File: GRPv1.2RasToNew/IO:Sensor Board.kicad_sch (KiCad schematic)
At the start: 20 parts, among them J1 B3B-XH-A, J3 B6B-XH-A, J4 B2B-XH-A, U1 BMP581, U2 ESP32-S3-DEVKITC-1-N8R2, U3 TPS79333-EP, U4 ICM-20948, U5 TPS79318-EP

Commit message: teensy modification
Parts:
- removed Module1: ComputeModule4-CM4, CM4IO:Raspberry-Pi-4-Compute-Module, symbol CM4IO:ComputeModule4-CM4
- removed U2: ESP32-S3-DEVKITC-1-N8R2, ESP32-S3-DEVKITC-1-N8R2:XCVR_ESP32-S3-DEVKITC-1-N8R2, symbol ESP32-S3-DEVKITC-1-N8R2:ESP32-S3-DEVKITC-1-N8R2
- added U6: Teensy4.1, modFiles:Teensy41, symbol teensy:Teensy4.1
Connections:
- net +5V: now also U6.48 (VIN)
- net BMP_CLK: now also U6.19 (27_A13_SCK1)
- net BMP_CS: now also U6.2 (0_RX1_CRX2_CS1)
- net BMP_MISO: now also U6.3 (1_TX1_CTX2_MISO1)
- net BMP_MOSI: now also U6.18 (26_A12_MOSI1)
- net GND: now also U6.1 (GND), U6.34 (GND), U6.47 (GND), U6.52 (GND), U6.58 (GND), U6.59 (GND), U6.64 (GND)
- net ICM_CLK: now also U6.35 (13_SCK_LED)
- net ICM_CS: now also U6.29 (37_CS)
- net ICM_MISO: now also U6.14 (12_MISO_MQSL)
- net ICM_MOSI: now also U6.13 (11_MOSI_CTX1)
- net PYRO_1: now also U6.27 (35_TX8)
- net PYRO_2: now also U6.26 (34_RX8)
- net PYRO_3: now also U6.25 (33_MCLK2)
- net PYRO_4: now also U6.39 (17_A3_TX4_SDA1)
- net PYRO_5: now also U6.38 (16_A2_RX4_SCL1)
- net SERVO_1: now also U6.45 (23_A9_CRX1_MCLK1)
- net SERVO_2: now also U6.44 (22_A8_CTX1)
- net SERVO_3: now also U6.41 (19_A5_SCL)
- net SERVO_4: now also U6.40 (18_A4_SDA)

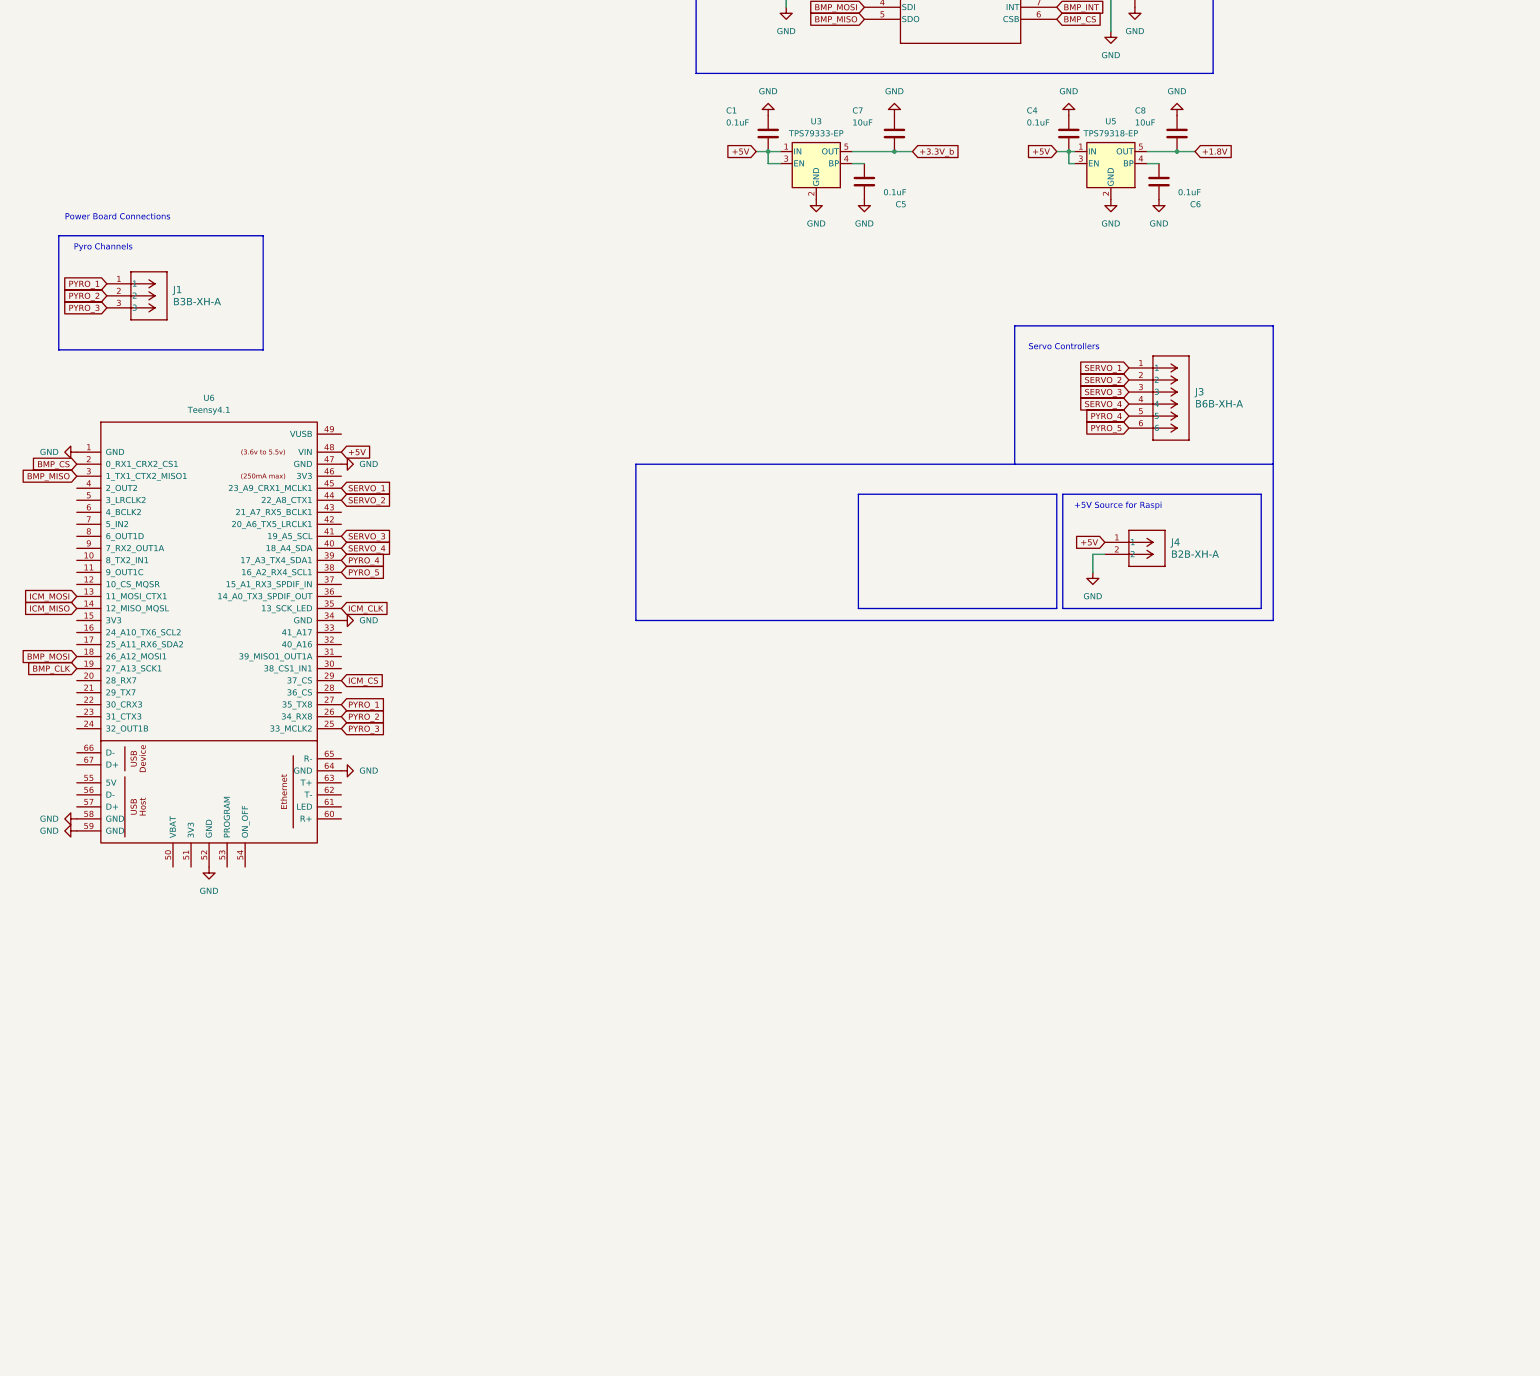
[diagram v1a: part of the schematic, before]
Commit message: esp switch 1
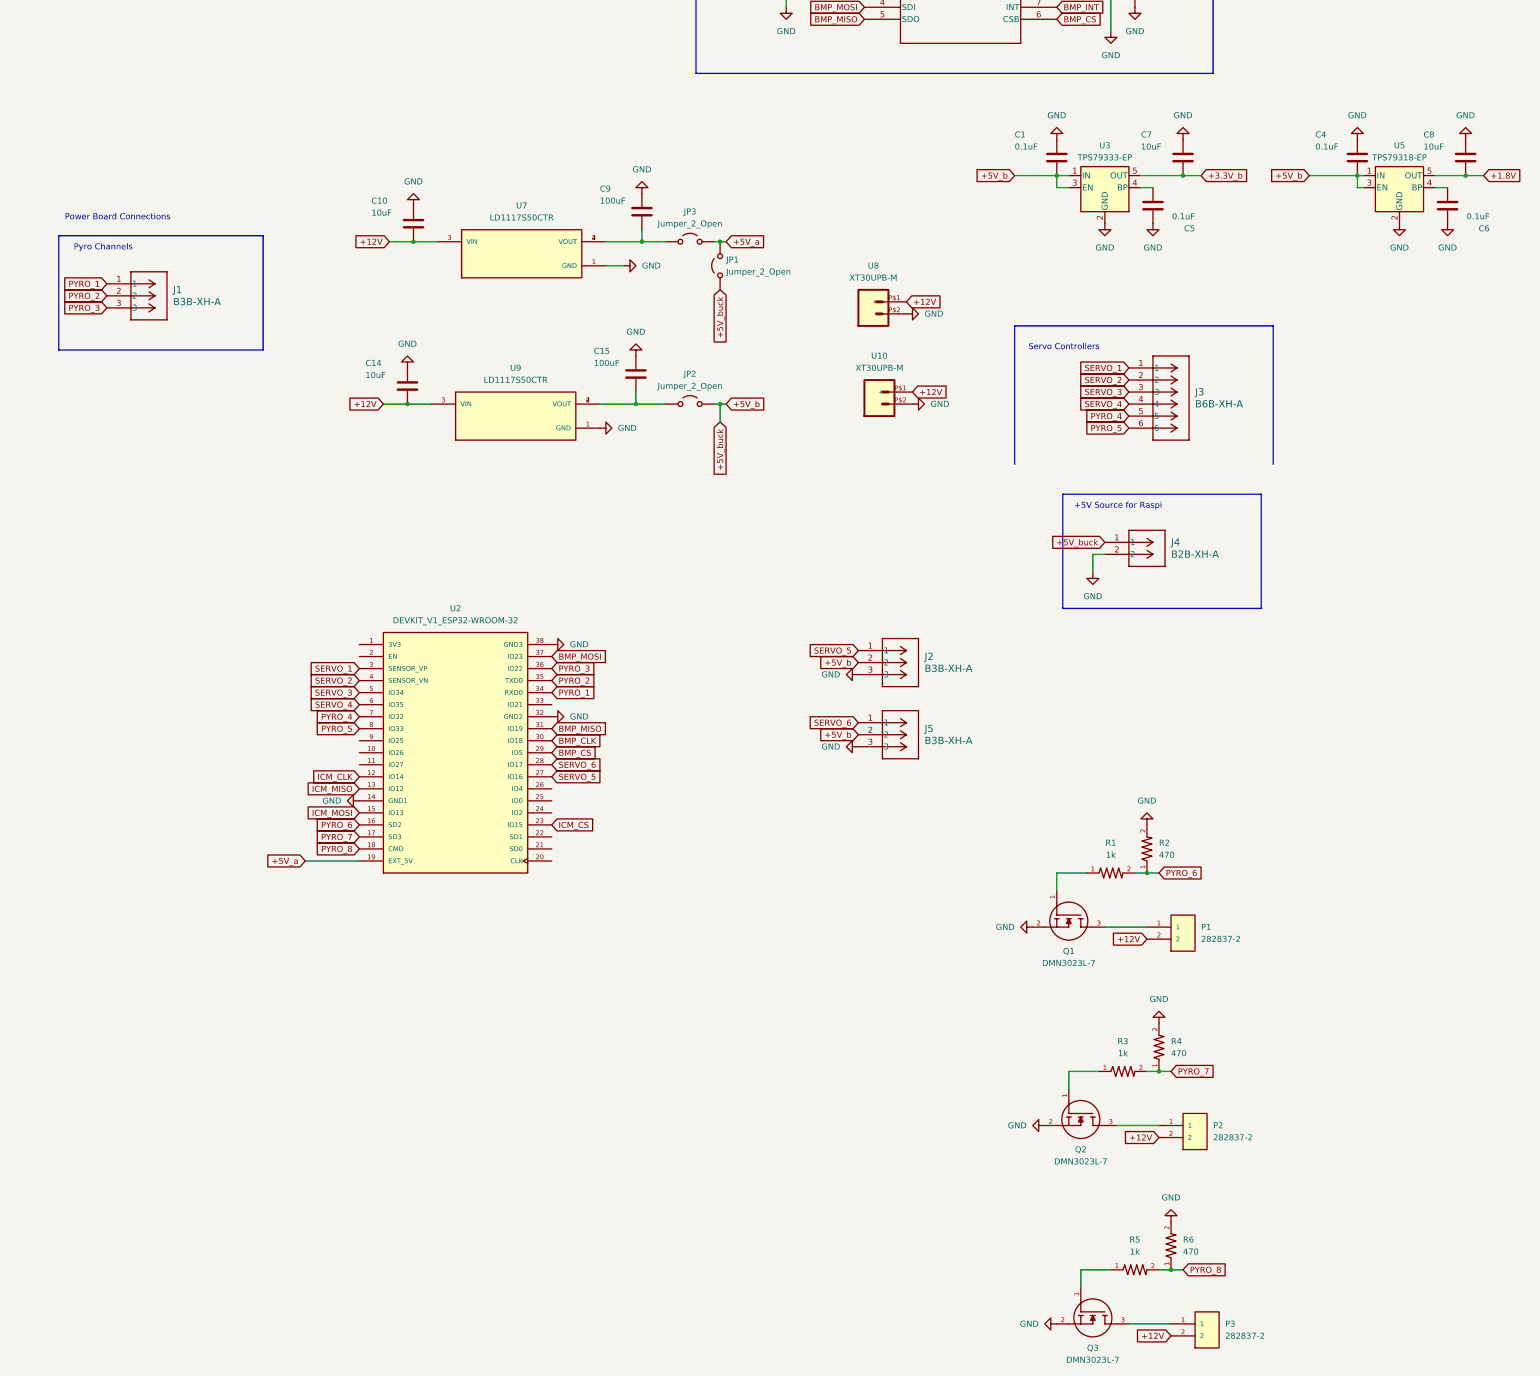
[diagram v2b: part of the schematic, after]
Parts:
- removed U6: Teensy4.1, modFiles:Teensy41, symbol teensy:Teensy4.1
- added C10, C14: 10uF, Capacitors:C_0805_2012Metric_Pad1.18x1.45mm_HandSolder, symbol Device:C
- added C15, C9: 100uF, Capacitors:C_0805_2012Metric_Pad1.18x1.45mm_HandSolder, symbol Device:C
- added J2, J5: B3B-XH-A, B3B:CONN_B3B-XH-A_JST, symbol 2025-01-01_02-21-05:B3B-XH-A
- added JP1, JP2, JP3: Jumper_2_Open, Jumper:SolderJumper-2_P1.3mm_Open_RoundedPad1.0x1.5mm, symbol Jumper:Jumper_2_Open
- added P1, P2, P3: 282837-2, ScrewTerminal:CUI_TB002-500-02BE, symbol 282837-2:282837-2
- added Q1, Q2, Q3: DMN3023L-7, FETS:SOT96P240X100-3N, symbol DMN3023L-7:DMN3023L-7
- added R1, R3, R5: 1k, Resistor:R_0805_2012Metric_Pad1.20x1.40mm_HandSolder, symbol 8-2176243-2:8-2176243-2
- added R2, R4, R6: 470, Resistor:R_0805_2012Metric_Pad1.20x1.40mm_HandSolder, symbol 8-2176243-2:8-2176243-2
- added U10, U8: XT30UPB-M, XTConnectors:XT30UPB-M, symbol XT30UPB-M:XT30UPB-M
- added U2: DEVKIT_V1_ESP32-WROOM-32, esp32wroom:MODULE_DEVKIT_V1_ESP32-WROOM-32, symbol DEVKIT_V1_ESP32-WROOM-32:DEVKIT_V1_ESP32-WROOM-32
- added U7, U9: LD1117S50CTR, LD1117S50CTRlib:LD1117S50CTR, symbol LD1117S50CTR:LD1117S50CTR
- C1, C11, C12, C13, C2, C3, C4, C5, C6, C7, C8: footprint Capacitor_SMD:C_0805_2012Metric_Pad1.18x1.45mm_HandSolder -> Capacitors:C_0805_2012Metric_Pad1.18x1.45mm_HandSolder
- J1: footprint Connector_JST:JST_XH_B3B-XH-A_1x03_P2.50mm_Vertical -> B3B:CONN_B3B-XH-A_JST
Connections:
- net BMP_CLK: now also U2.30 (IO18)
- net BMP_CS: now also U2.29 (IO5)
- net BMP_MISO: now also U2.31 (IO19)
- net BMP_MOSI: now also U2.37 (IO23)
- net GND: now also C10.1, C14.1, C15.1, C9.1, J2.3, J5.3, Q1.2, Q2.2, Q3.2, R2.2, R4.2, R6.2, U10.P$2 (-), U2.14 (GND1), U2.32 (GND2), U2.38 (GND3), U7.1 (GND), U8.P$2 (-), U9.1 (GND)
- net ICM_CLK: now also U2.12 (IO14)
- net ICM_CS: now also U2.23 (IO15)
- net ICM_MISO: now also U2.13 (IO12)
- net ICM_MOSI: now also U2.15 (IO13)
- net PYRO_1: now also U2.34 (RXD0)
- net PYRO_2: now also U2.35 (TXD0)
- net PYRO_3: now also U2.36 (IO22)
- net PYRO_4: now also U2.7 (IO32)
- net PYRO_5: now also U2.8 (IO33)
- net SERVO_1: now also U2.3 (SENSOR_VP)
- net SERVO_2: now also U2.4 (SENSOR_VN)
- net SERVO_3: now also U2.5 (IO34)
- net SERVO_4: now also U2.6 (IO35)
- net +5V renamed +5V_b
- net +5V_b: now also J2.2, J5.2, JP1.1 (A), JP2.2 (B)
- new net: Q1.1, R1.1
- new net: P1.1, Q1.3
- new net: Q2.1, R3.1
- new net: P2.1, Q2.3
- new net: C15.2, JP2.1 (A), U9.2 (VOUT), U9.4 (VOUT)
- new net: C9.2, JP3.1 (A), U7.2 (VOUT), U7.4 (VOUT)
- new net: P3.1, Q3.3
- new net: Q3.1, R5.1
- new net +12V: C10.2, C14.2, P1.2, P2.2, P3.2, U10.P$1 (+), U7.3 (VIN), U8.P$1 (+), U9.3 (VIN)
- new net +5V_a: JP1.2 (B), JP3.2 (B), U2.19 (EXT_5V)
- new net PYRO_6: R1.2, R2.1, U2.16 (SD2)
- new net PYRO_7: R3.2, R4.1, U2.17 (SD3)
- new net PYRO_8: R5.2, R6.1, U2.18 (CMD)
- new net SERVO_5: J2.1, U2.27 (IO16)
- new net SERVO_6: J5.1, U2.28 (IO17)
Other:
- moved on the sheet: C1, C4, C5, C6, C7, C8, U3, U5

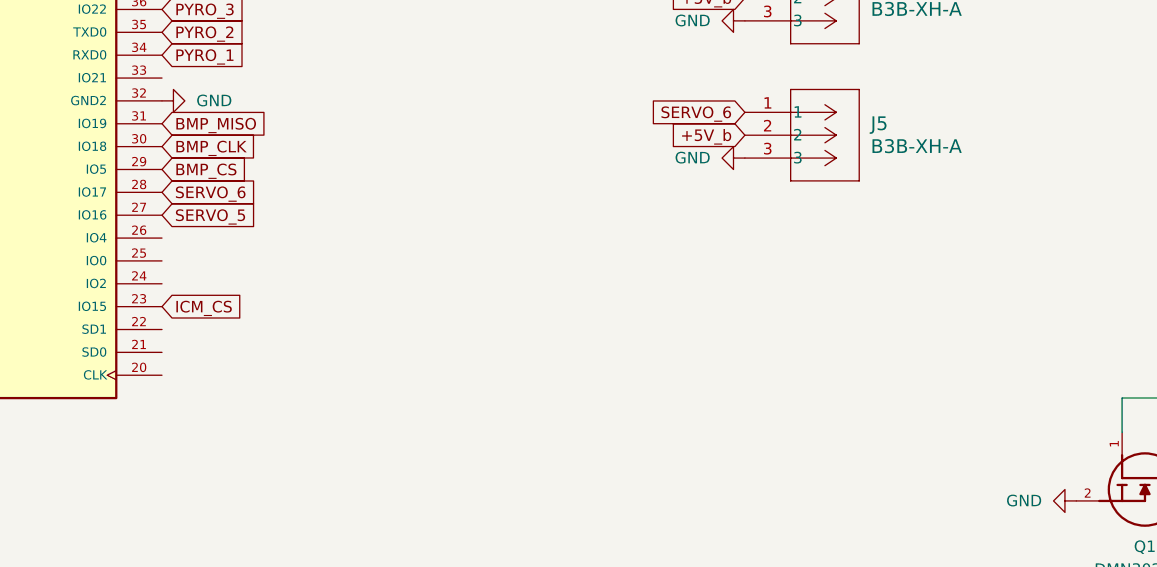
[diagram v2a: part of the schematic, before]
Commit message: checkoff with pwm
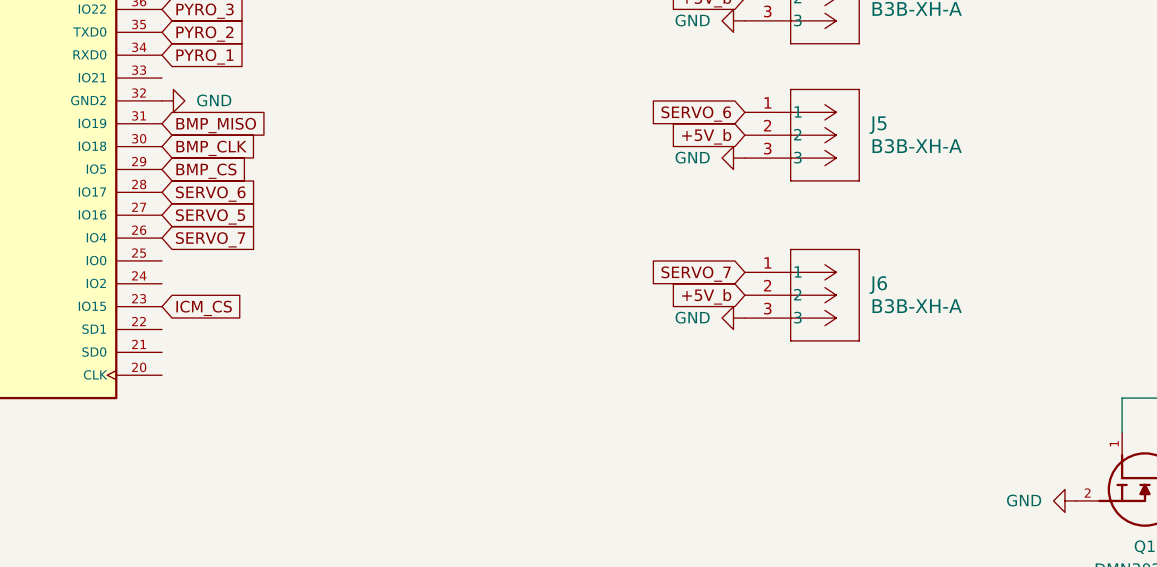
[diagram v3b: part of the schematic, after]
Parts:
- added J6: B3B-XH-A, NewJST:CONN_B3B-XH-A_JST, symbol 2025-01-01_02-21-05:B3B-XH-A
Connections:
- net +5V_b: now also J6.2
- net GND: now also J6.3
- net SERVO_7: now reaches U2.26 (IO4)
- net SERVO_7: now also J6.1
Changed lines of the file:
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@@
 		)
 	)
+	(global_label "SERVO_7"
+		(shape input)
+		(at 139.7 283.21 0)
+		(fields_autoplaced yes)
+		(effects
+			(font
+				(size 1.27 1.27)
+			)
+			(justify left)
+		)
+		(property "Intersheetrefs" "${INTERSHEET_REFS}"
+			(at 150.9099 283.21 0)
+			(effects
+				(font
+					(size 1.27 1.27)
+				)
+				(justify left)
+				(hide yes)
+			)
+		)
+	)
 	(global_label "+5V_a"
 		(shape input)
@@
 		)
 	)
+	(global_label "+5V_b"
+		(shape input)
+		(at 204.47 289.56 180)
+		(fields_autoplaced yes)
+		(effects
+			(font
+				(size 1.27 1.27)
+			)
+			(justify right)
+		)
+		(property "Intersheetrefs" "${INTERSHEET_REFS}"
+			(at 195.4977 289.56 0)
+			(effects
+				(font
+					(size 1.27 1.27)
+				)
+				(justify right)
+				(hide yes)
+			)
+		)
+	)
 	(global_label "ICM_MISO"
 		(shape input)
@@
 		)
 	)
+	(global_label "SERVO_7"
+		(shape input)
+		(at 204.47 287.02 180)
+		(fields_autoplaced yes)
+		(effects
+			(font
+				(size 1.27 1.27)
+			)
+			(justify right)
+		)
+		(property "Intersheetrefs" "${INTERSHEET_REFS}"
+			(at 193.2601 287.02 0)
+			(effects
+				(font
+					(size 1.27 1.27)
+				)
+				(justify right)
+				(hide yes)
+			)
+		)
+	)
 	(global_label "+5V_a"
 		(shape input)
@@
 	)
 	(symbol
+		(lib_id "power:GND")
+		(at 204.47 292.1 270)
+		(unit 1)
+		(exclude_from_sim no)
+		(in_bom yes)
+		(on_board yes)
+		(dnp no)
+		(fields_autoplaced yes)
+		(property "Reference" "#PWR060"
+			(at 198.12 292.1 0)
+			(effects
+				(font
+					(size 1.27 1.27)
+				)
+				(hide yes)
+			)
+		)
+		(property "Value" "GND"
+			(at 200.66 292.0999 90)
+			(effects
+				(font
+					(size 1.27 1.27)
+				)
+				(justify right)
+			)
+		)
+		(property "Footprint" ""
+			(at 204.47 292.1 0)
+			(effects
+				(font
+					(size 1.27 1.27)
+				)
+				(hide yes)
+			)
+		)
+		(property "Datasheet" ""
+			(at 204.47 292.1 0)
+			(effects
+				(font
+					(size 1.27 1.27)
+				)
+				(hide yes)
+			)
+		)
+		(property "Description" "Power symbol creates a global label with name \"GND\" , ground"
+			(at 204.47 292.1 0)
+			(effects
+				(font
+					(size 1.27 1.27)
+				)
+				(hide yes)
+			)
+		)
+		(pin "1"
+		)
+		(instances
+			(project "IO:Sensor Board"
+				(path "/18c0d8c9-9c3d-4e29-9dd2-642815852ae9"
+					(reference "#PWR060")
+					(unit 1)
+				)
+			)
+		)
+	)
+	(symbol
 		(lib_id "Device:C")
 		(at 158.75 48.26 0)
@@
 					(unit 1)
 				)
+			)
+		)
+	)
+	(symbol
+		(lib_id "2025-01-01_02-21-05:B3B-XH-A")
+		(at 204.47 287.02 0)
+		(unit 1)
+		(exclude_from_sim no)
+		(in_bom yes)
+		(on_board yes)
+		(dnp no)
+		(fields_autoplaced yes)
+		(property "Reference" "J6"
+			(at 218.44 288.2899 0)
+			(effects
+				(font
+					(size 1.524 1.524)
+				)
+				(justify left)
+			)
+		)
+		(property "Value" "B3B-XH-A"
+			(at 218.44 290.8299 0)
+			(effects
+				(font
+					(size 1.524 1.524)
+				)
+				(justify left)
+			)
+		)
+		(property "Footprint" "NewJST:CONN_B3B-XH-A_JST"
+			(at 204.47 287.02 0)
+			(effects
+				(font
+					(size 1.27 1.27)
+					(italic yes)
+				)
+				(hide yes)
+			)
+		)
+		(property "Datasheet" "B3B-XH-A"
+			(at 204.47 287.02 0)
+			(effects
+				(font
+					(size 1.27 1.27)
+					(italic yes)
+				)
+				(hide yes)
+			)
+		)
+		(property "Description" ""
+			(at 204.47 287.02 0)
+			(effects
+				(font
+					(size 1.27 1.27)
+				)
+				(hide yes)
+			)
+		)
+		(pin "3"
+		)
+		(pin "2"
+		)
+		(pin "1"
+		)
+		(instances
+			(project "IO:Sensor Board"
+				(path "/18c0d8c9-9c3d-4e29-9dd2-642815852ae9"
+					(reference "J6")
+					(unit 1)
+				)
